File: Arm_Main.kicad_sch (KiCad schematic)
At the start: 58 parts, among them IC1 TLP559_F_, IC2 TLP559_F_, J1 Conn_01x02_Pin, J2 Conn_01x03_Socket, J3 Conn_01x03_Pin, J4 Conn_01x03_Pin, J5 Conn_01x03_Pin, SW1 SW_SPST, SW2 SW_SPST, SW3 SW_SPST, U1 ADuM121N, U2 TLP2531, U3 RASPBERRY_PI_ZERO_2_W, U4 LM350_TO220

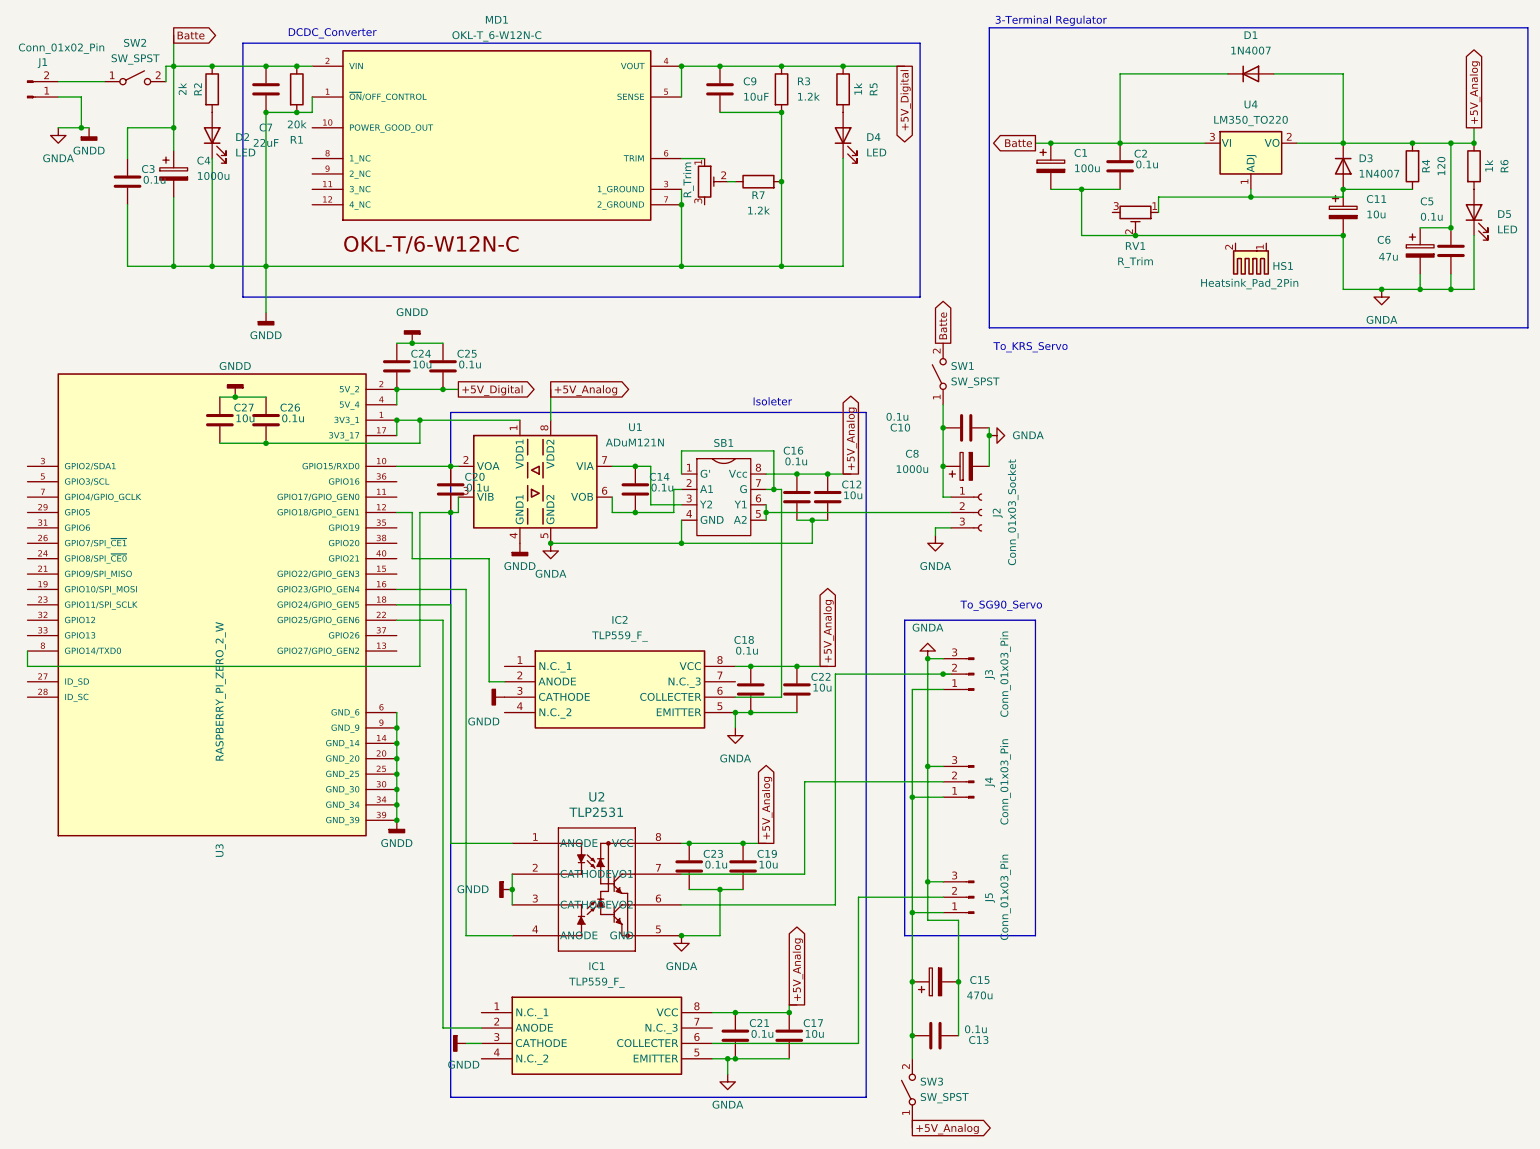
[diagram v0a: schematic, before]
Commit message: ver10.1
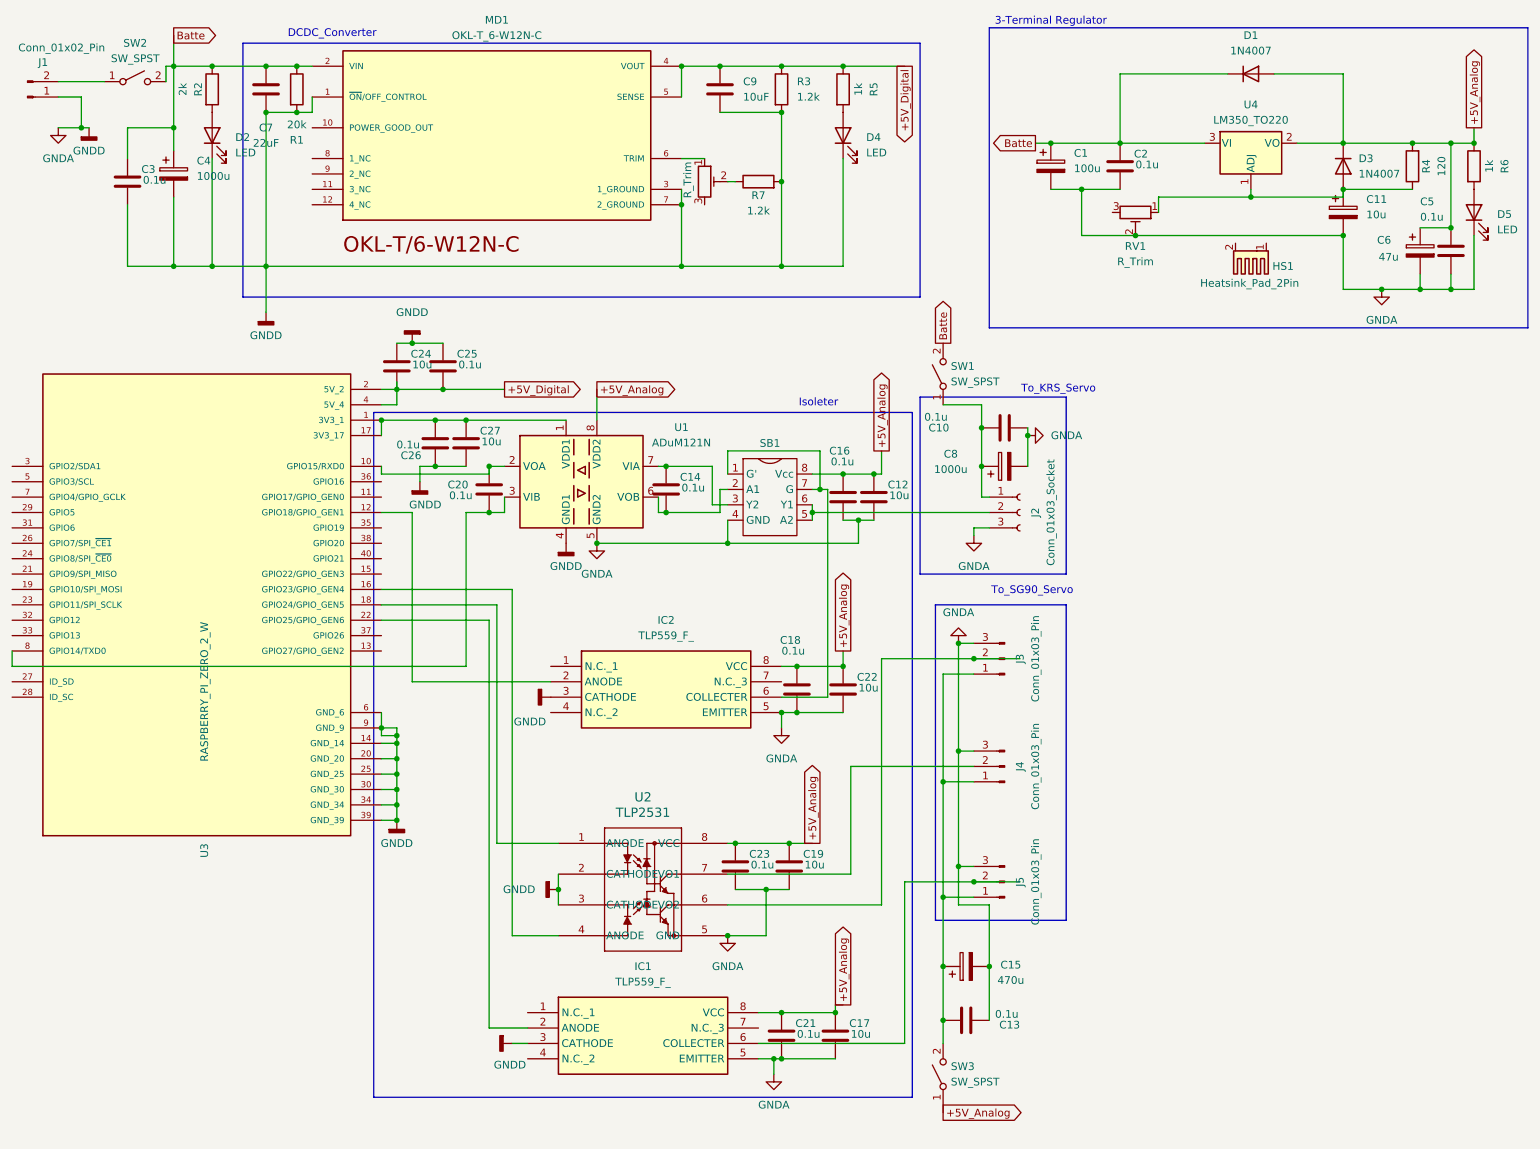
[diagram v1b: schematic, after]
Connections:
- net GNDA: now also C27.2; no longer C27.1
- net at C26.2, U1.1 (VDD1), U3.1 (3V3_1)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: now also C27.1; no longer C27.2
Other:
- moved on the sheet: C10, C12, C13, C14, C15, C16, C17, C18, C19, C20, C21, C22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
